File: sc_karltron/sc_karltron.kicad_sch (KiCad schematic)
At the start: 38 parts, among them J1 Conn_01x02, J2 Conn_01x02, U1 TL074, U2 TL074

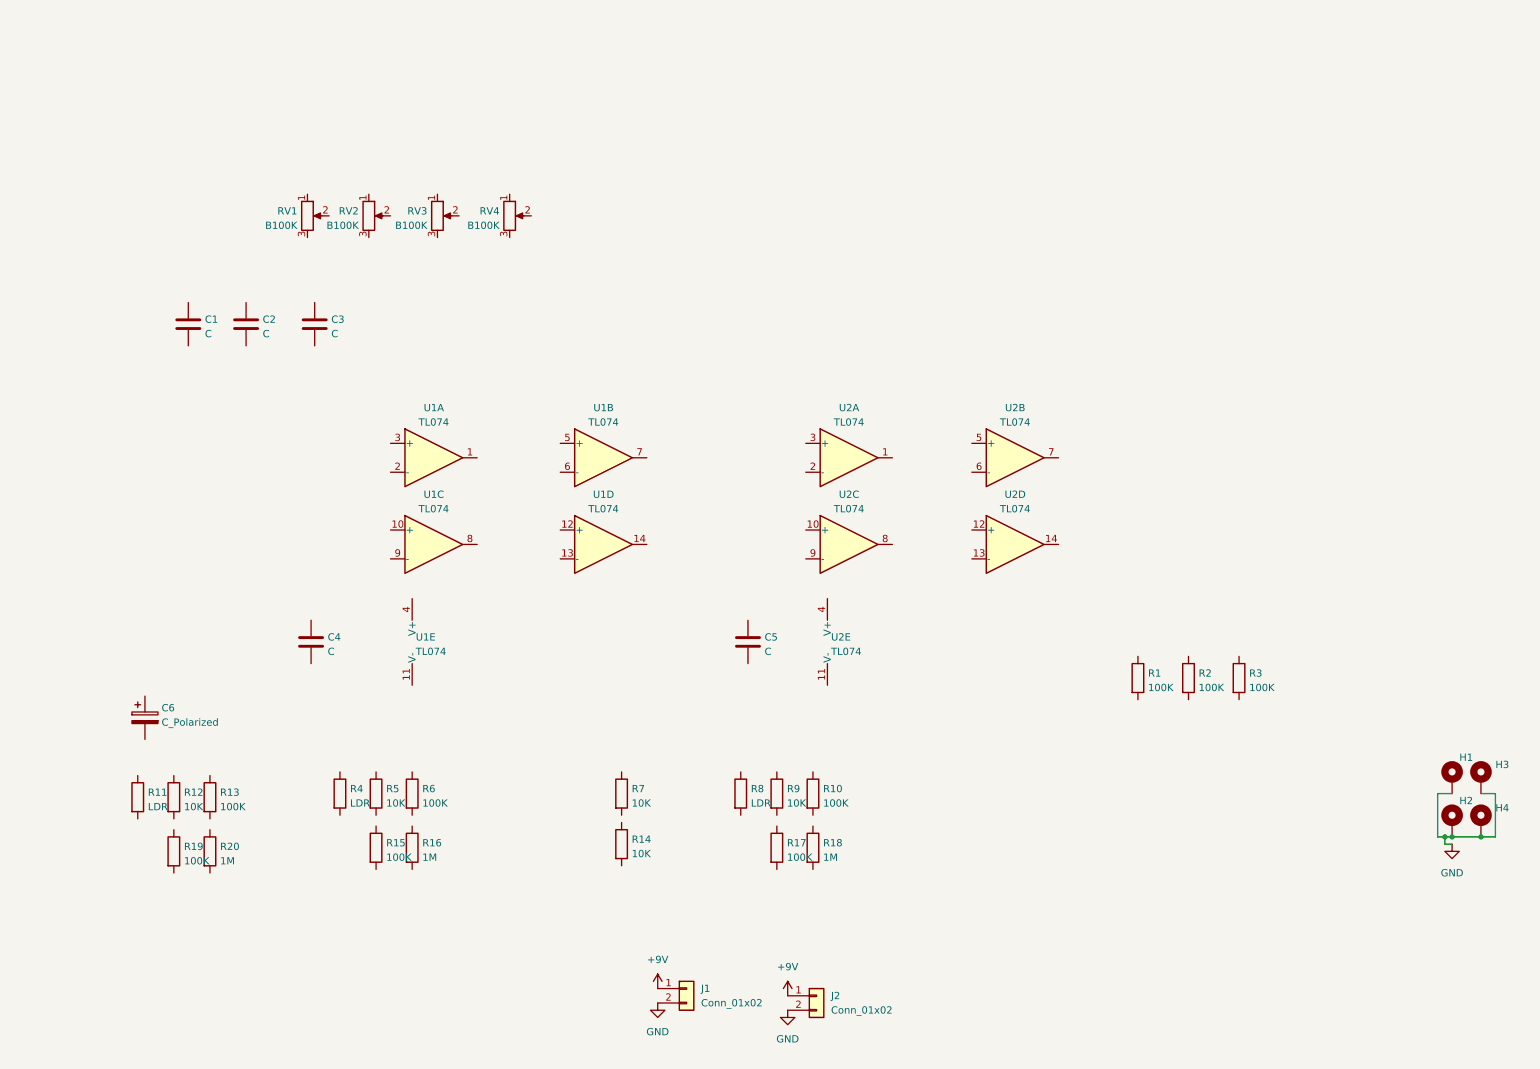
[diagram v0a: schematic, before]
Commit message: working too
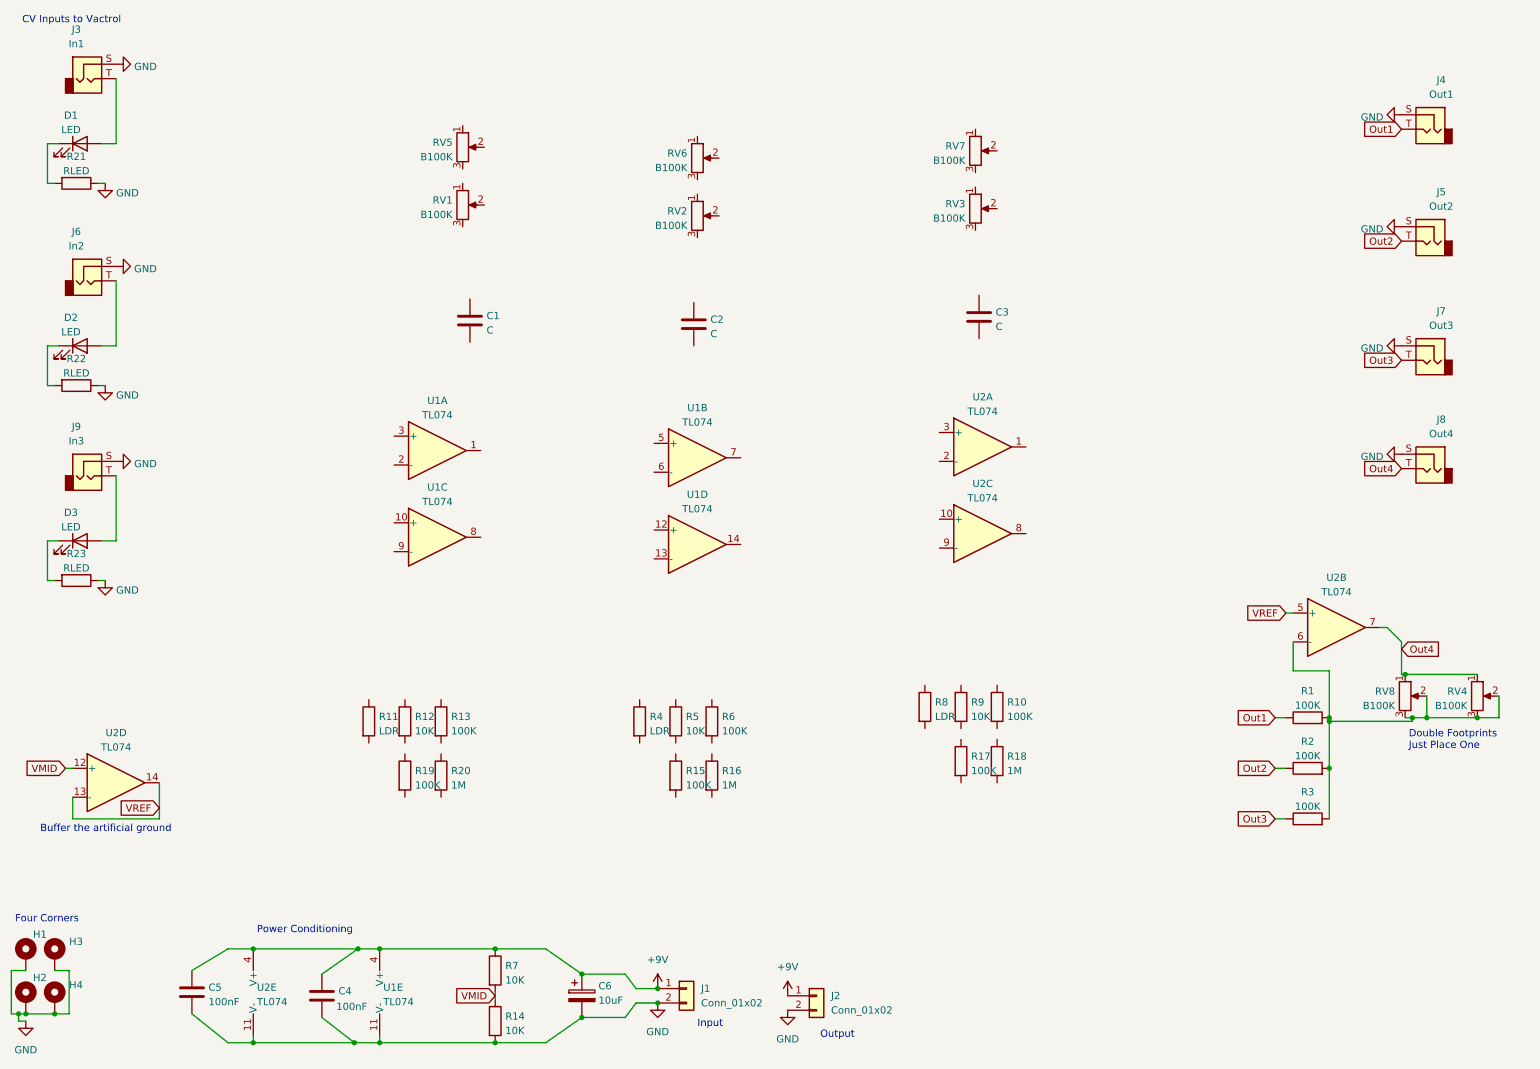
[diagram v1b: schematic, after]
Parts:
- added D1, D2, D3: LED, LED_THT:LED_D5.0mm_Horizontal_O3.81mm_Z3.0mm, symbol Device:LED
- added J3: In1, Connector_PinHeader_2.54mm:PinHeader_1x02_P2.54mm_Vertical, symbol Connector:AudioJack2
- added J4: Out1, Connector_PinHeader_2.54mm:PinHeader_1x02_P2.54mm_Vertical, symbol Connector:AudioJack2
- added J5: Out2, Connector_PinHeader_2.54mm:PinHeader_1x02_P2.54mm_Vertical, symbol Connector:AudioJack2
- added J6: In2, Connector_PinHeader_2.54mm:PinHeader_1x02_P2.54mm_Vertical, symbol Connector:AudioJack2
- added J7: Out3, Connector_PinHeader_2.54mm:PinHeader_1x02_P2.54mm_Vertical, symbol Connector:AudioJack2
- added J8: Out4, Connector_PinHeader_2.54mm:PinHeader_1x02_P2.54mm_Vertical, symbol Connector:AudioJack2
- added J9: In3, Connector_PinHeader_2.54mm:PinHeader_1x02_P2.54mm_Vertical, symbol Connector:AudioJack2
- added R21, R22, R23: RLED, Resistor_THT:R_Axial_DIN0207_L6.3mm_D2.5mm_P10.16mm_Horizontal, symbol Device:R
- added RV5, RV6, RV7, RV8: B100K, Potentiometer_THT:Potentiometer_Alpha_RD901F-40-00D_Single_Vertical, symbol Device:R_Potentiometer
- C4, C5: value C -> 100nF
- C6: value C_Polarized -> 10uF
- RV1, RV2, RV3, RV4: footprint Potentiometer_THT:Potentiometer_ACP_CA9-V10_Vertical -> Potentiometer_THT:Potentiometer_ACP_CA9-H5_Horizontal
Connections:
- net +9V: now also C4.1, C5.1, C6.1, R7.1, U1.4 (V+), U2.4 (V+)
- net GND: now also C4.2, C5.2, C6.2, R14.2, U1.11 (V-), U2.11 (V-), J3.S, J4.S, J5.S, J6.S, J7.S, J8.S, J9.S, R21.1, R22.1, R23.1
- net Out2: now reaches R2.1
- net Out2: now also J5.T
- net at R2.2: now also R1.2, R3.2, RV4.2, RV4.3, U2.6 (-), RV8.2, RV8.3
- net VMID: now reaches R14.1
- net VMID: now also R7.2, U2.12 (+)
- net Out4: now reaches RV4.1
- net Out4: now also U2.7, J8.T, RV8.1
- net Out3: now reaches R3.1
- net Out3: now also J7.T
- net VREF: now reaches U2.13 (-)
- net VREF: now also U2.14, U2.5 (+)
- net Out1: now reaches R1.1
- net Out1: now also J4.T
- new net: D2.2 (A), J6.T
- new net: D2.1 (K), R22.2
- new net: D1.2 (A), J3.T
- new net: D1.1 (K), R21.2
- new net: D3.2 (A), J9.T
- new net: D3.1 (K), R23.2
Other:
- note added: "Buffer the artificial ground"
- note added: "CV Inputs to Vactrol"
- note added: "Double Footprints Just Place One"
- note added: "Four Corners"
- note added: "Input"
- note added: "Output"
- note added: "Power Conditioning"
- company: (none) -> Karltron
- title: (none) -> Synthcard:Karltron
- moved on the sheet: C1, C2, C3, C4, C5, C6, H1, H2, H3, H4, R1, R10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
